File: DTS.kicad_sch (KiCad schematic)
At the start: 9 parts, among them J4 Conn_01x06_Pin, J5 Conn_01x02_Pin, J6 Conn_01x02_Pin, J7 Conn_01x06_Pin, SW1 SW_DIP_x01, U23 4069, U69 LM7805_TO220

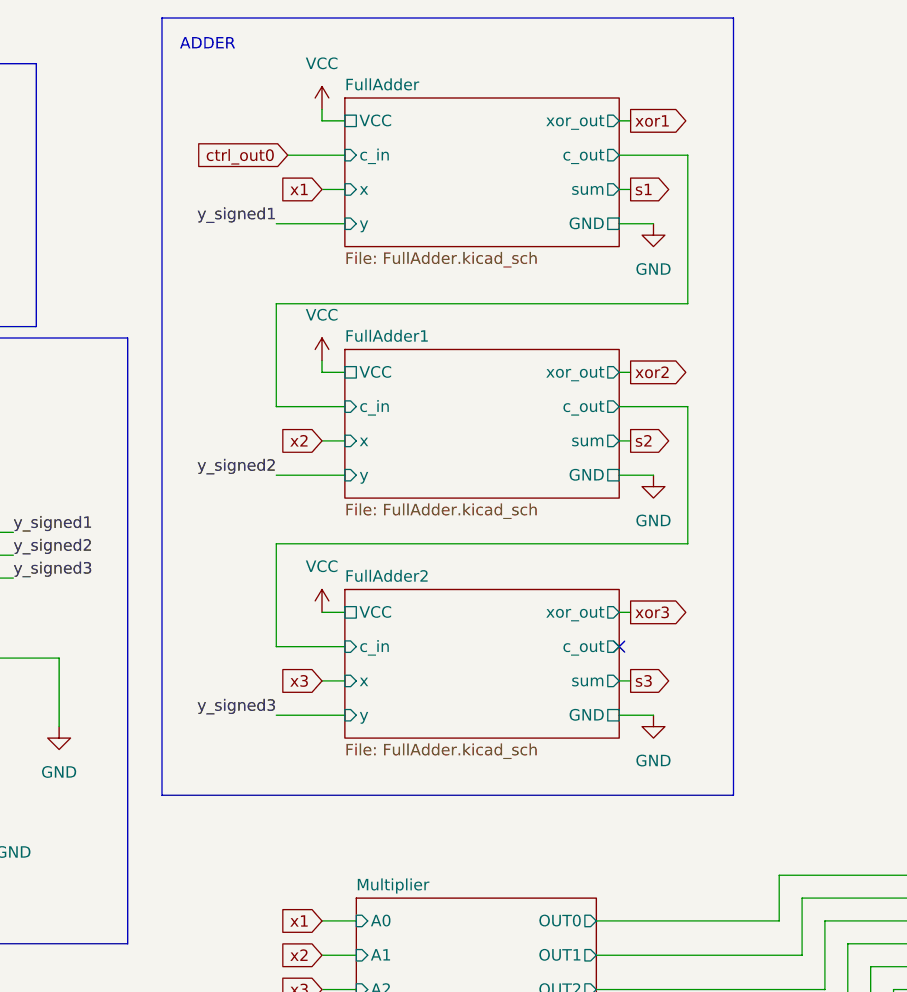
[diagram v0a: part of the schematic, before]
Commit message: Add files via upload
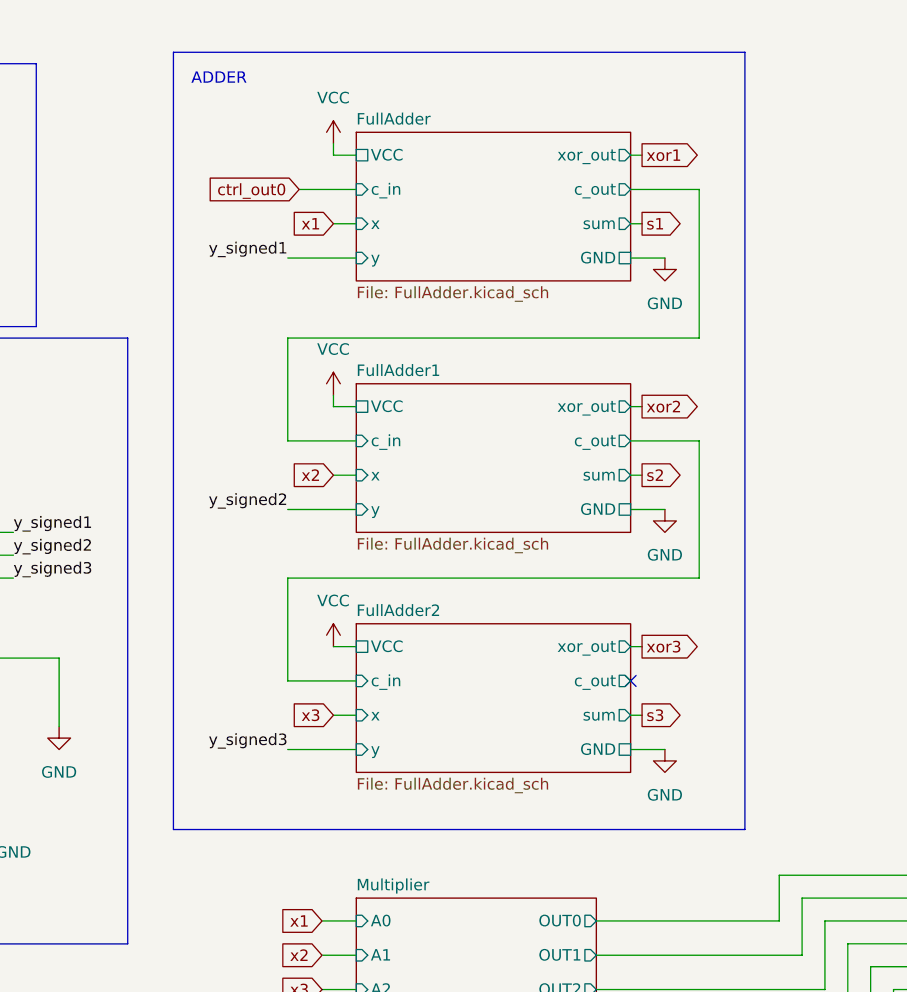
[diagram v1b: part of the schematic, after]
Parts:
- C1, C2: footprint (none) -> Capacitor_THT:C_Rect_L7.0mm_W2.0mm_P5.00mm
- J4, J7: footprint (none) -> Connector_PinHeader_2.54mm:PinHeader_1x06_P2.54mm_Vertical
- J5, J6: footprint (none) -> Connector_PinHeader_2.54mm:PinHeader_1x02_P2.54mm_Vertical
- SW1: footprint (none) -> Connector_PinSocket_2.54mm:PinSocket_1x02_P2.54mm_Vertical
- U23: footprint (none) -> Package_DIP:CERDIP-14_W7.62mm_SideBrazed_LongPads_Socket
